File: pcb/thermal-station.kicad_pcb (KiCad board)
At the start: 2 copper layers, 107.9 x 64.2 mm, 38 parts, among them J1 Jack-DC, J2 Conn_01x03, J3 Conn_01x04_Male, Q1 AO3401A, SW1 RESET, SW2 SW_DIP_x02, SW3 FLASH, U1 ESP-12E, U10 KCSA02-105, U11 KCSA02-105, U12 DS18B20, U2 74HC595, U3 74HC595, U4 KCSA02-105, U5 KCSA02-105, U6 MH-Z19, U7 LM1117-3.3, U8 74HC595, U9 74HC595

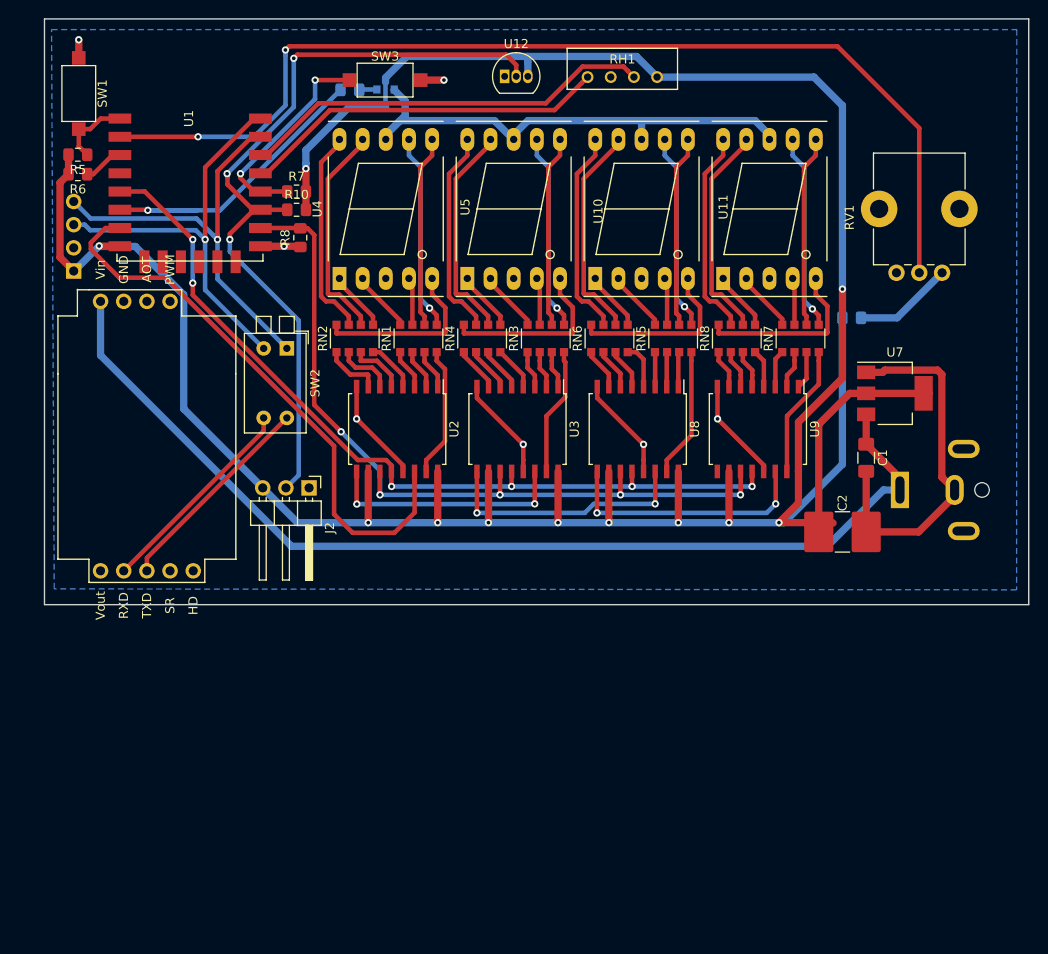
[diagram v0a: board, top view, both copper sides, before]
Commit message: Redesign PCB
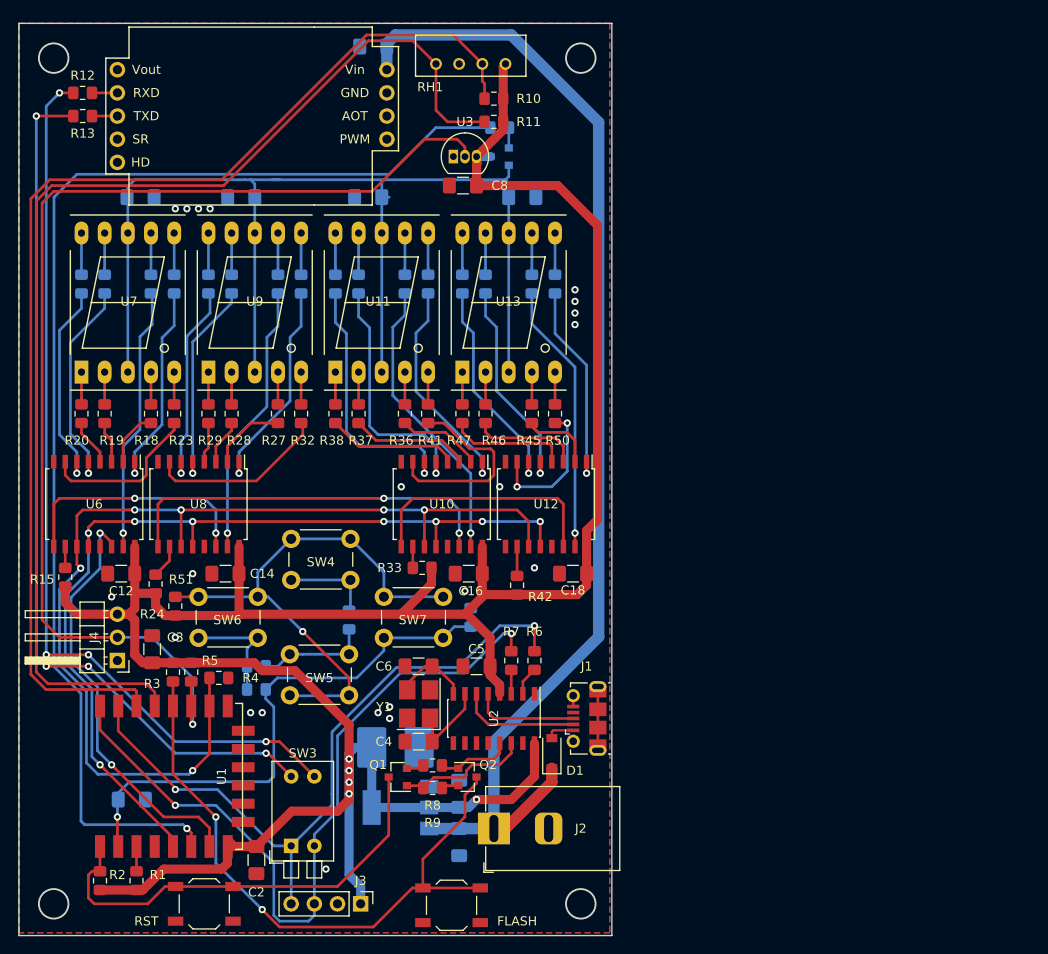
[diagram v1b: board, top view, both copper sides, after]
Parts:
- removed RN1, RN2, RN3, RN4, RN5, RN6, RN7, RN8: R_Pack04, Resistor_SMD:R_Array_Convex_4x1206
- removed RV1: R_POT, Potentiometer_THT:Potentiometer_Alps_RK09K_Single_Vertical
- removed SW1: RESET, Button_Switch_SMD:SW_SPST_CK_RS282G05A3
- removed SW2: SW_DIP_x02, Button_Switch_THT:SW_DIP_SPSTx02_Piano_10.8x6.64mm_W7.62mm_P2.54mm
- added C10: 10uF, Capacitor_SMD:C_1206_3216Metric_Pad1.42x1.75mm_HandSolder, B.Cu at (163.2, 139.8)
- added C11: 100uF, Capacitor_SMD:C_2816_7142Metric_Pad3.20x4.45mm_HandSolder, B.Cu at (156.2, 129.4)
- added C12: 0.1uF, Capacitor_SMD:C_1206_3216Metric_Pad1.42x1.75mm_HandSolder, F.Cu at (126.2, 110.3)
- added C13: 0.1uF, Capacitor_SMD:C_1206_3216Metric_Pad1.42x1.75mm_HandSolder, B.Cu at (128.3, 69.1)
- added C14: 0.1uF, Capacitor_SMD:C_1206_3216Metric_Pad1.42x1.75mm_HandSolder, F.Cu at (137.6, 110.3)
- added C15: 0.1uF, Capacitor_SMD:C_1206_3216Metric_Pad1.42x1.75mm_HandSolder, B.Cu at (139.3, 69.1)
- added C16: 0.1uF, Capacitor_SMD:C_1206_3216Metric_Pad1.42x1.75mm_HandSolder, F.Cu at (164.3, 110.3)
- added C17: 0.1uF, Capacitor_SMD:C_1206_3216Metric_Pad1.42x1.75mm_HandSolder, B.Cu at (153.2, 69.1)
- added C18: 0.1uF, Capacitor_SMD:C_1206_3216Metric_Pad1.42x1.75mm_HandSolder, F.Cu at (175.7, 110.3)
- added C19: 0.1uF, Capacitor_SMD:C_1206_3216Metric_Pad1.42x1.75mm_HandSolder, B.Cu at (170.1, 69.1)
- added C3: 0.1uF, Capacitor_SMD:C_1206_3216Metric_Pad1.42x1.75mm_HandSolder, F.Cu at (129.6, 118.6)
- added C4: 22pF, Capacitor_SMD:C_1206_3216Metric_Pad1.42x1.75mm_HandSolder, F.Cu at (158.8, 128.8)
- added C5: 10uF, Capacitor_SMD:C_1206_3216Metric_Pad1.42x1.75mm_HandSolder, F.Cu at (165.1, 120.5)
- added C6: 22pF, Capacitor_SMD:C_1206_3216Metric_Pad1.42x1.75mm_HandSolder, F.Cu at (158.8, 120.5)
- added C7: 10uF, Capacitor_SMD:C_1206_3216Metric_Pad1.42x1.75mm_HandSolder, B.Cu at (163.2, 134.5)
- added C8: 0.1uF, Capacitor_SMD:C_1206_3216Metric_Pad1.42x1.75mm_HandSolder, F.Cu at (163.6, 67.8)
- added C9: 0.1uF, Capacitor_SMD:C_1206_3216Metric_Pad1.42x1.75mm_HandSolder, B.Cu at (153.8, 52.6)
- added D1: B240A-E3, Diode_SMD:D_SOD-123, F.Cu at (173.4, 130.0)
- added FLASH: FLASH, Button_Switch_SMD:SW_SPST_TL3342, F.Cu at (162.4, 146.7)
- added J4: Conn_01x03, Connector_PinHeader_2.54mm:PinHeader_1x03_P2.54mm_Horizontal, F.Cu at (125.7, 119.9)
- added Q2: S8050, Package_TO_SOT_SMD:SOT-23, F.Cu at (164.1, 132.6)
- added Q3: IRLML2502, Package_TO_SOT_SMD:SOT-23, B.Cu at (167.7, 64.6)
- added R11: 2K2, Resistor_SMD:R_0805_2012Metric_Pad1.15x1.40mm_HandSolder, F.Cu at (167.0, 60.8)
- added R12: 4K7, Resistor_SMD:R_0805_2012Metric_Pad1.15x1.40mm_HandSolder, F.Cu at (121.9, 57.6)
- added R13: 4K7, Resistor_SMD:R_0805_2012Metric_Pad1.15x1.40mm_HandSolder, F.Cu at (121.9, 60.2)
- added R14: 1K, Resistor_SMD:R_0805_2012Metric_Pad1.15x1.40mm_HandSolder, B.Cu at (167.7, 61.4)
- added R15: 1K, Resistor_SMD:R_0805_2012Metric_Pad1.15x1.40mm_HandSolder, F.Cu at (120.0, 110.7)
- added R16: 160, Resistor_SMD:R_0805_2012Metric_Pad1.15x1.40mm_HandSolder, B.Cu at (129.4, 78.6)
- added R17: 160, Resistor_SMD:R_0805_2012Metric_Pad1.15x1.40mm_HandSolder, B.Cu at (132.0, 78.6)
- added R18: 160, Resistor_SMD:R_0805_2012Metric_Pad1.15x1.40mm_HandSolder, F.Cu at (129.4, 92.8)
- added R19: 160, Resistor_SMD:R_0805_2012Metric_Pad1.15x1.40mm_HandSolder, F.Cu at (124.4, 92.8)
- added R2: 10K, Resistor_SMD:R_0805_2012Metric_Pad1.15x1.40mm_HandSolder, F.Cu at (123.8, 144.0)
- added R20: 160, Resistor_SMD:R_0805_2012Metric_Pad1.15x1.40mm_HandSolder, F.Cu at (121.8, 92.8)
- added R21: 160, Resistor_SMD:R_0805_2012Metric_Pad1.15x1.40mm_HandSolder, B.Cu at (124.4, 78.6)
- added R22: 160, Resistor_SMD:R_0805_2012Metric_Pad1.15x1.40mm_HandSolder, B.Cu at (121.8, 78.6)
- added R23: 160, Resistor_SMD:R_0805_2012Metric_Pad1.15x1.40mm_HandSolder, F.Cu at (132.0, 92.8)
- added R24: 1K, Resistor_SMD:R_0805_2012Metric_Pad1.15x1.40mm_HandSolder, F.Cu at (129.9, 111.5)
- added R25: 160, Resistor_SMD:R_0805_2012Metric_Pad1.15x1.40mm_HandSolder, B.Cu at (143.3, 78.6)
- added R26: 160, Resistor_SMD:R_0805_2012Metric_Pad1.15x1.40mm_HandSolder, B.Cu at (145.9, 78.6)
- added R27: 160, Resistor_SMD:R_0805_2012Metric_Pad1.15x1.40mm_HandSolder, F.Cu at (143.3, 92.8)
- added R28: 160, Resistor_SMD:R_0805_2012Metric_Pad1.15x1.40mm_HandSolder, F.Cu at (138.3, 92.8)
- added R29: 160, Resistor_SMD:R_0805_2012Metric_Pad1.15x1.40mm_HandSolder, F.Cu at (135.7, 92.8)
- added R3: 10K, Resistor_SMD:R_0805_2012Metric_Pad1.15x1.40mm_HandSolder, F.Cu at (131.8, 121.1)
- added R30: 160, Resistor_SMD:R_0805_2012Metric_Pad1.15x1.40mm_HandSolder, B.Cu at (138.3, 78.6)
- added R31: 160, Resistor_SMD:R_0805_2012Metric_Pad1.15x1.40mm_HandSolder, B.Cu at (135.7, 78.6)
- added R32: 160, Resistor_SMD:R_0805_2012Metric_Pad1.15x1.40mm_HandSolder, F.Cu at (145.9, 92.8)
- added R33: 1K, Resistor_SMD:R_0805_2012Metric_Pad1.15x1.40mm_HandSolder, F.Cu at (159.2, 109.7)
- added R34: 160, Resistor_SMD:R_0805_2012Metric_Pad1.15x1.40mm_HandSolder, B.Cu at (157.3, 78.6)
- added R35: 160, Resistor_SMD:R_0805_2012Metric_Pad1.15x1.40mm_HandSolder, B.Cu at (159.8, 78.6)
- added R36: 160, Resistor_SMD:R_0805_2012Metric_Pad1.15x1.40mm_HandSolder, F.Cu at (157.3, 92.8)
- added R37: 160, Resistor_SMD:R_0805_2012Metric_Pad1.15x1.40mm_HandSolder, F.Cu at (152.2, 92.8)
- added R38: 160, Resistor_SMD:R_0805_2012Metric_Pad1.15x1.40mm_HandSolder, F.Cu at (149.6, 92.8)
- added R39: 160, Resistor_SMD:R_0805_2012Metric_Pad1.15x1.40mm_HandSolder, B.Cu at (152.2, 78.6)
- added R4: 10K, Resistor_SMD:R_0805_2012Metric_Pad1.15x1.40mm_HandSolder, F.Cu at (136.9, 121.8)
- added R40: 160, Resistor_SMD:R_0805_2012Metric_Pad1.15x1.40mm_HandSolder, B.Cu at (149.6, 78.6)
- added R41: 160, Resistor_SMD:R_0805_2012Metric_Pad1.15x1.40mm_HandSolder, F.Cu at (159.8, 92.8)
- added R42: 1K, Resistor_SMD:R_0805_2012Metric_Pad1.15x1.40mm_HandSolder, F.Cu at (169.6, 111.6)
- added R43: 160, Resistor_SMD:R_0805_2012Metric_Pad1.15x1.40mm_HandSolder, B.Cu at (171.2, 78.6)
- added R44: 160, Resistor_SMD:R_0805_2012Metric_Pad1.15x1.40mm_HandSolder, B.Cu at (173.7, 78.6)
- added R45: 160, Resistor_SMD:R_0805_2012Metric_Pad1.15x1.40mm_HandSolder, F.Cu at (171.2, 92.8)
- added R46: 160, Resistor_SMD:R_0805_2012Metric_Pad1.15x1.40mm_HandSolder, F.Cu at (166.1, 92.8)
- added R47: 160, Resistor_SMD:R_0805_2012Metric_Pad1.15x1.40mm_HandSolder, F.Cu at (163.6, 92.8)
- added R48: 160, Resistor_SMD:R_0805_2012Metric_Pad1.15x1.40mm_HandSolder, B.Cu at (166.1, 78.6)
- added R49: 160, Resistor_SMD:R_0805_2012Metric_Pad1.15x1.40mm_HandSolder, B.Cu at (163.6, 78.6)
- added R50: 160, Resistor_SMD:R_0805_2012Metric_Pad1.15x1.40mm_HandSolder, F.Cu at (173.7, 92.8)
- added R51: 56K, Resistor_SMD:R_0805_2012Metric_Pad1.15x1.40mm_HandSolder, F.Cu at (132.1, 113.9)
- added R52: 56K, Resistor_SMD:R_0805_2012Metric_Pad1.15x1.40mm_HandSolder, B.Cu at (151.1, 115.4)
- added R53: 56K, Resistor_SMD:R_0805_2012Metric_Pad1.15x1.40mm_HandSolder, B.Cu at (141.0, 120.5)
- added R54: 56K, Resistor_SMD:R_0805_2012Metric_Pad1.15x1.40mm_HandSolder, B.Cu at (141.0, 123.0)
- added R55: 56K, Resistor_SMD:R_0805_2012Metric_Pad1.15x1.40mm_HandSolder, B.Cu at (164.5, 115.1)
- added RST: RESET, Button_Switch_SMD:SW_SPST_TL3342, F.Cu at (135.3, 146.5)
- added SW4: BRIGHT UP, Button_Switch_THT:SW_PUSH_6mm_H8.5mm, F.Cu at (144.8, 106.5)
- added SW5: BRIGHT DOWN, Button_Switch_THT:SW_PUSH_6mm_H8.5mm, F.Cu at (151.1, 123.7)
- added SW6: NEXT, Button_Switch_THT:SW_PUSH_6mm_H8.5mm, F.Cu at (134.6, 112.9)
- added SW7: PREV, Button_Switch_THT:SW_PUSH_6mm_H8.5mm, F.Cu at (155.0, 112.9)
- added U13: KCSA02-105, Display_7Segment:7SegmentLED_LTS6760_LTS6780, F.Cu at (163.6, 88.2)
- added Y1: HC-49, Crystal:Crystal_SMD_SeikoEpson_FA238V-4Pin_3.2x2.5mm_HandSoldering, F.Cu at (158.8, 124.6)
- C1: value C -> 0.1uF; moved to B.Cu
- C2: value CP -> 0.1uF; footprint Capacitor_SMD:C_2816_7142Metric_Pad3.20x4.45mm_HandSolder -> Capacitor_SMD:C_1206_3216Metric_Pad1.42x1.75mm_HandSolder
- J1: value Jack-DC -> USB; footprint Connector_BarrelJack:BarrelJack_CUI_PJ-063AH_Horizontal -> Connector_USB:USB_Micro-B_Molex-105017-0001; moved to F.Cu
- J2: value Conn_01x03 -> Jack-DC; footprint Connector_PinHeader_2.54mm:PinHeader_1x03_P2.54mm_Horizontal -> Connector_BarrelJack:BarrelJack_Horizontal_DS_201
- J3: moved to F.Cu
- Q1: value AO3401A -> S8050; moved to F.Cu
- R1, R9: value R -> 10K; moved to F.Cu
- R10: value R -> 2K2
- R5, R8: value R -> 10K
- R6, R7: value R -> 470
- SW3: value FLASH -> SW_DIP_x02; footprint Button_Switch_SMD:SW_SPST_CK_RS282G05A3 -> Button_Switch_THT:SW_DIP_SPSTx02_Piano_10.8x6.64mm_W7.62mm_P2.54mm
- U10: value KCSA02-105 -> 74HC595; footprint Display_7Segment:7SegmentLED_LTS6760_LTS6780 -> Package_SO:SOIC-16W_7.5x10.3mm_P1.27mm
- U12: value DS18B20 -> 74HC595; footprint Package_TO_SOT_THT:TO-92_Inline -> Package_SO:SOIC-16W_7.5x10.3mm_P1.27mm
- U2: value 74HC595 -> CH340G; footprint Package_SO:SOIC-16W_7.5x10.3mm_P1.27mm -> Package_SO:SOIC-16_3.9x9.9mm_P1.27mm
- U3: value 74HC595 -> DS18B20; footprint Package_SO:SOIC-16W_7.5x10.3mm_P1.27mm -> Package_TO_SOT_THT:TO-92_Inline
- U4: value KCSA02-105 -> MH-Z19; footprint Display_7Segment:7SegmentLED_LTS6760_LTS6780 -> mh-z19:MH-Z19
- U5: value KCSA02-105 -> LM1117-3.3; footprint Display_7Segment:7SegmentLED_LTS6760_LTS6780 -> Package_TO_SOT_SMD:SOT-223-3_TabPin2; moved to B.Cu
- U6: value MH-Z19 -> 74HC595; footprint mh-z19:MH-Z19 -> Package_SO:SOIC-16W_7.5x10.3mm_P1.27mm
- U7: value LM1117-3.3 -> KCSA02-105; footprint Package_TO_SOT_SMD:SOT-223-3_TabPin2 -> Display_7Segment:7SegmentLED_LTS6760_LTS6780
- U9: value 74HC595 -> KCSA02-105; footprint Package_SO:SOIC-16W_7.5x10.3mm_P1.27mm -> Display_7Segment:7SegmentLED_LTS6760_LTS6780
- moved R1 89.8 mm to (127.8, 144.0), turned to 270 degrees
- moved U7 89.2 mm to (121.8, 88.2), turned to 90 degrees
- moved C1 88.8 mm to (127.3, 135.1), turned to 0 degrees
- moved SW3 84.6 mm to (144.8, 140.2), turned to 90 degrees
- moved U1 79.2 mm to (123.8, 139.6), turned to 90 degrees
- moved J3 76.2 mm to (152.4, 146.5), turned to 270 degrees
- moved Q1 74.4 mm to (156.5, 132.6), turned to 180 degrees
- moved C2 73.6 mm to (141.0, 141.7), turned to 270 degrees
- moved R6 73.1 mm to (171.5, 119.9), turned to 270 degrees
- moved R9 69.0 mm to (160.3, 133.8)
- moved U9 60.6 mm to (135.7, 88.2), turned to 90 degrees
- moved R8 59.6 mm to (160.3, 131.4), turned to 0 degrees
- moved U5 58.5 mm to (156.8, 136.0), turned to 180 degrees
- moved R5 58.1 mm to (133.8, 121.1), turned to 90 degrees
- moved R7 56.5 mm to (168.9, 119.9), turned to 270 degrees
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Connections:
- C1 pad 1: +5V -> ADC
- J1 pad 1: +5V -> Net-(D1-Pad2)
- J1 pad 2: Earth -> Net-(J1-Pad2)
- J2 pad 1: Earth -> +5V
- J2 pad 2: 1WIRE -> Earth
- J3 pad 3: TX -> TXD
- J3 pad 4: RX -> RXD
- Q1 pad 3: +3V3 -> RST
- R1 pad 1: PWM -> Net-(R1-Pad1)
- R1 pad 2: Net-(Q1-Pad1) -> +3V3
- R10 pad 1: 1WIRE -> +3V3
- R10 pad 2: +3V3 -> SDA
- R5 pad 1: Net-(R5-Pad1) -> 1WIRE
- R6 pad 1: Net-(R6-Pad1) -> RXD
- R6 pad 2: +3V3 -> Net-(R6-Pad2)
- R7 pad 1: Net-(R7-Pad1) -> TXD
- R7 pad 2: +3V3 -> Net-(R7-Pad2)
- R8 pad 1: Earth -> Net-(Q1-Pad2)
- R8 pad 2: SS -> Net-(Q2-Pad1)
- R9 pad 2: +3V3 -> Net-(Q1-Pad1)
- SW3 pad 1: Net-(R7-Pad1) -> RXD
- SW3 pad 2: Earth -> TXD
- U1 pad 1: Net-(R5-Pad1) -> RST
- U1 pad 12: Net-(R7-Pad1) -> GPIO0
- U1 pad 15: RX -> RXD
- U1 pad 16: TX -> TXD
- U1 pad 3: Net-(R6-Pad1) -> Net-(R1-Pad1)
- U10 pad 1: Net-(RN6-Pad5) -> /DISPLAY/LED_3/QB
- U10 pad 2: Net-(RN5-Pad8) -> /DISPLAY/LED_3/QC
- U10 pad 3: Net-(U10-Pad3) -> /DISPLAY/LED_3/QD
- U10 pad 4: Net-(RN5-Pad7) -> /DISPLAY/LED_3/QE
- U10 pad 5: Net-(RN6-Pad8) -> /DISPLAY/LED_3/QF
- U10 pad 6: Net-(RN5-Pad6) -> /DISPLAY/LED_3/QG
- U10 pad 7: Net-(RN5-Pad5) -> /DISPLAY/LED_3/QH
- U10 pad 8: Net-(Q1-Pad2) -> Earth
- U10 pad 9: Net-(RN6-Pad6) -> /DISPLAY/LED_4/DATA_IN
- U11 pad 3: Net-(U11-Pad3) -> LED_CA
- U11 pad 8: Net-(Q1-Pad2) -> LED_CA
- U12 pad 1: Earth -> /DISPLAY/LED_4/QB
- U12 pad 2: 1WIRE -> /DISPLAY/LED_4/QC
- U12 pad 3: +3V3 -> /DISPLAY/LED_4/QD
- U2 pad 1: Net-(RN1-Pad3) -> Earth
- U2 pad 10: +3V3 -> Net-(U2-Pad10)
- U2 pad 11: SS -> Net-(U2-Pad11)
- U2 pad 12: Clock -> Net-(U2-Pad12)
- U2 pad 13: Earth -> Net-(Q2-Pad1)
- U2 pad 14: MOSI -> Net-(Q1-Pad1)
- U2 pad 2: Net-(RN1-Pad2) -> Net-(R6-Pad2)
- U2 pad 3: Net-(RN1-Pad1) -> Net-(R7-Pad2)
- U2 pad 4: Net-(RN2-Pad4) -> +3V3
- U2 pad 5: Net-(RN2-Pad3) -> Net-(J1-Pad3)
- U2 pad 6: Net-(RN2-Pad2) -> Net-(J1-Pad2)
- U2 pad 8: Earth -> Net-(C6-Pad1)
- U3 pad 1: Net-(RN3-Pad3) -> Earth
- U3 pad 2: Net-(RN3-Pad2) -> 1WIRE
- U3 pad 3: Net-(RN3-Pad1) -> +3V3
- U4 pad 6: Net-(RN1-Pad6) -> +5V
- U4 pad 7: Net-(RN1-Pad5) -> Earth
- U4 pad 8: Net-(Q1-Pad2) -> Net-(U4-Pad8)
- U5 pad 1: Net-(RN4-Pad5) -> Earth
- U5 pad 2: Net-(RN3-Pad8) -> +3V3
- U5 pad 3: Net-(U5-Pad3) -> +5V
- U6 pad 1: Net-(U6-Pad1) -> /DISPLAY/LED_1/QB
- U6 pad 2: Net-(SW2-Pad3) -> /DISPLAY/LED_1/QC
- U6 pad 3: Net-(SW2-Pad4) -> /DISPLAY/LED_1/QD
- U6 pad 4: Net-(U6-Pad4) -> /DISPLAY/LED_1/QE
- U6 pad 5: Net-(U6-Pad5) -> /DISPLAY/LED_1/QF
- U6 pad 6: +5V -> /DISPLAY/LED_1/QG
- U6 pad 7: Earth -> /DISPLAY/LED_1/QH
- U6 pad 8: Net-(U6-Pad8) -> Earth
- U6 pad 9: Net-(U6-Pad9) -> /DISPLAY/LED_2/DATA_IN
- U7 pad 1: Earth -> Net-(R20-Pad1)
- U7 pad 2: +3V3 -> Net-(R19-Pad1)
- U7 pad 3: +5V -> LED_CA
- U8 pad 1: Net-(RN5-Pad3) -> /DISPLAY/LED_2/QB
- U8 pad 10: +3V3 -> Net-(R24-Pad2)
- U8 pad 14: Net-(U3-Pad9) -> /DISPLAY/LED_2/DATA_IN
- U8 pad 15: Net-(RN5-Pad4) -> /DISPLAY/LED_2/QA
- U8 pad 2: Net-(RN5-Pad2) -> /DISPLAY/LED_2/QC
- U8 pad 3: Net-(RN5-Pad1) -> /DISPLAY/LED_2/QD
- U8 pad 4: Net-(RN6-Pad4) -> /DISPLAY/LED_2/QE
- U8 pad 5: Net-(RN6-Pad3) -> /DISPLAY/LED_2/QF
- U8 pad 6: Net-(RN6-Pad2) -> /DISPLAY/LED_2/QG
- U8 pad 7: Net-(RN6-Pad1) -> /DISPLAY/LED_2/QH
- U8 pad 9: Net-(U8-Pad9) -> /DISPLAY/LED_3/DATA_IN
- U9 pad 10: +3V3 -> Net-(R31-Pad1)
- U9 pad 3: Net-(RN7-Pad1) -> LED_CA
- U9 pad 8: Earth -> LED_CA
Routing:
- net LED_CA: track 0.00 -> 129.1 mm
- net PWM: track 34.4 -> 134.0 mm
- net Net-(R12-Pad1): track 0.00 -> 98.6 mm, vias 0 -> 4
- net Net-(R13-Pad1): track 0.00 -> 96.7 mm, vias 0 -> 4
- net SCL: track 40.9 -> 130.8 mm
- net Earth: track 94.6 -> 7.00 mm, vias 7 -> 21
- net TXD: track 0.00 -> 84.1 mm, vias 0 -> 2
- net SDA: track 46.1 -> 129.0 mm
- net RXD: track 0.00 -> 76.9 mm, vias 0 -> 2
- net GPIO0: track 0.00 -> 70.1 mm, vias 0 -> 2
- net Net-(R51-Pad1): track 0.00 -> 59.9 mm, vias 0 -> 1
- net ADC: track 114.2 -> 59.1 mm, vias 2 -> 1
- net Net-(Q1-Pad2): track 54.8 -> 1.92 mm
- net RST: track 0.00 -> 50.1 mm
- net RX: track 45.6 -> 0.00 mm, vias 1 -> 0
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- added copper zone on F.Cu, net Earth
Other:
- board size 107.9 x 64.2 mm -> 65 x 100 mm
- net class 5V added: clearance 0.3, trace_width 1.25, via_dia 0.8, via_drill 0.4
- net class Default: clearance 0.25 -> 0.3; trace_width 0.25 -> 0.3
- net class Display added: clearance 0.3, trace_width 0.3, via_dia 0.8, via_drill 0.4
- net class Thin added: clearance 0.25, trace_width 0.25, via_dia 0.8, via_drill 0.4
- net class VCC added: clearance 0.3, trace_width 1, via_dia 0.8, via_drill 0.4
- rule trace_clearance: 0.25 -> 0.3
- board text added: "BRNV.RU"
- board text added: "REV 0.2"
- board text added: "THERMAL STATION"
